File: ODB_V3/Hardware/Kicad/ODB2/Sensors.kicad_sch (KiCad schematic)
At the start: 24 parts, among them J4 RF2-04A-T-00-50-G, U10 ADXL382-2BCCZ-RL7, U4 MS580301BA01-00, U5 L76L-M33, U6 BNO055, U9 MAX6612MXK

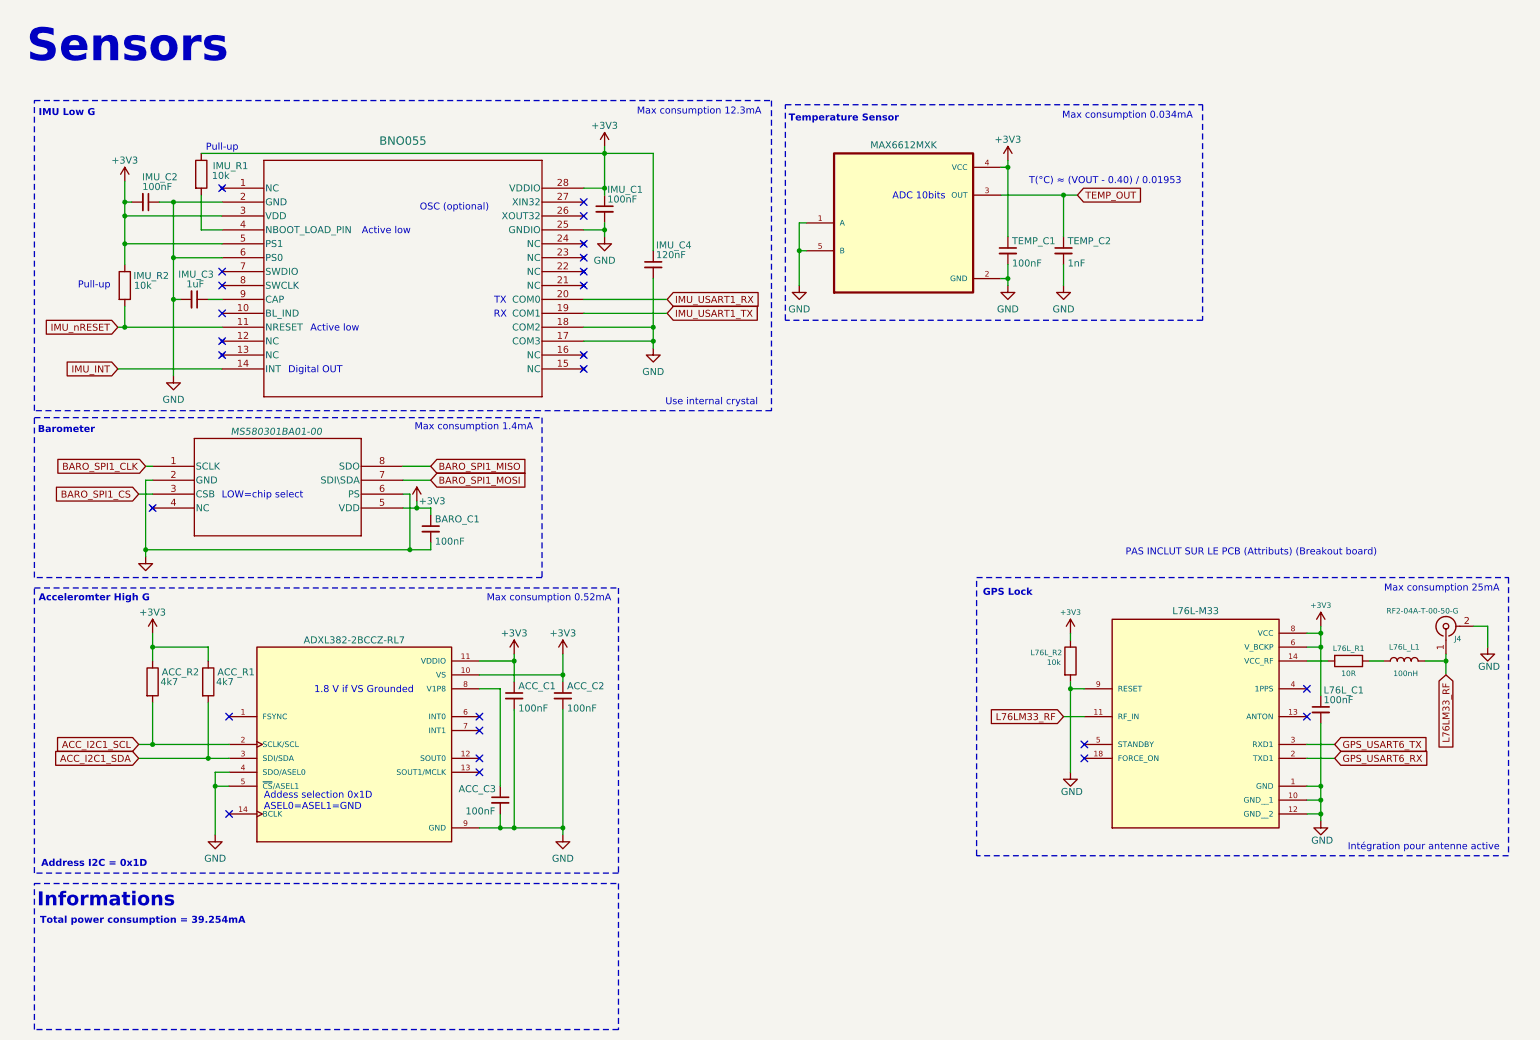
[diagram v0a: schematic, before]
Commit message: fix: labels
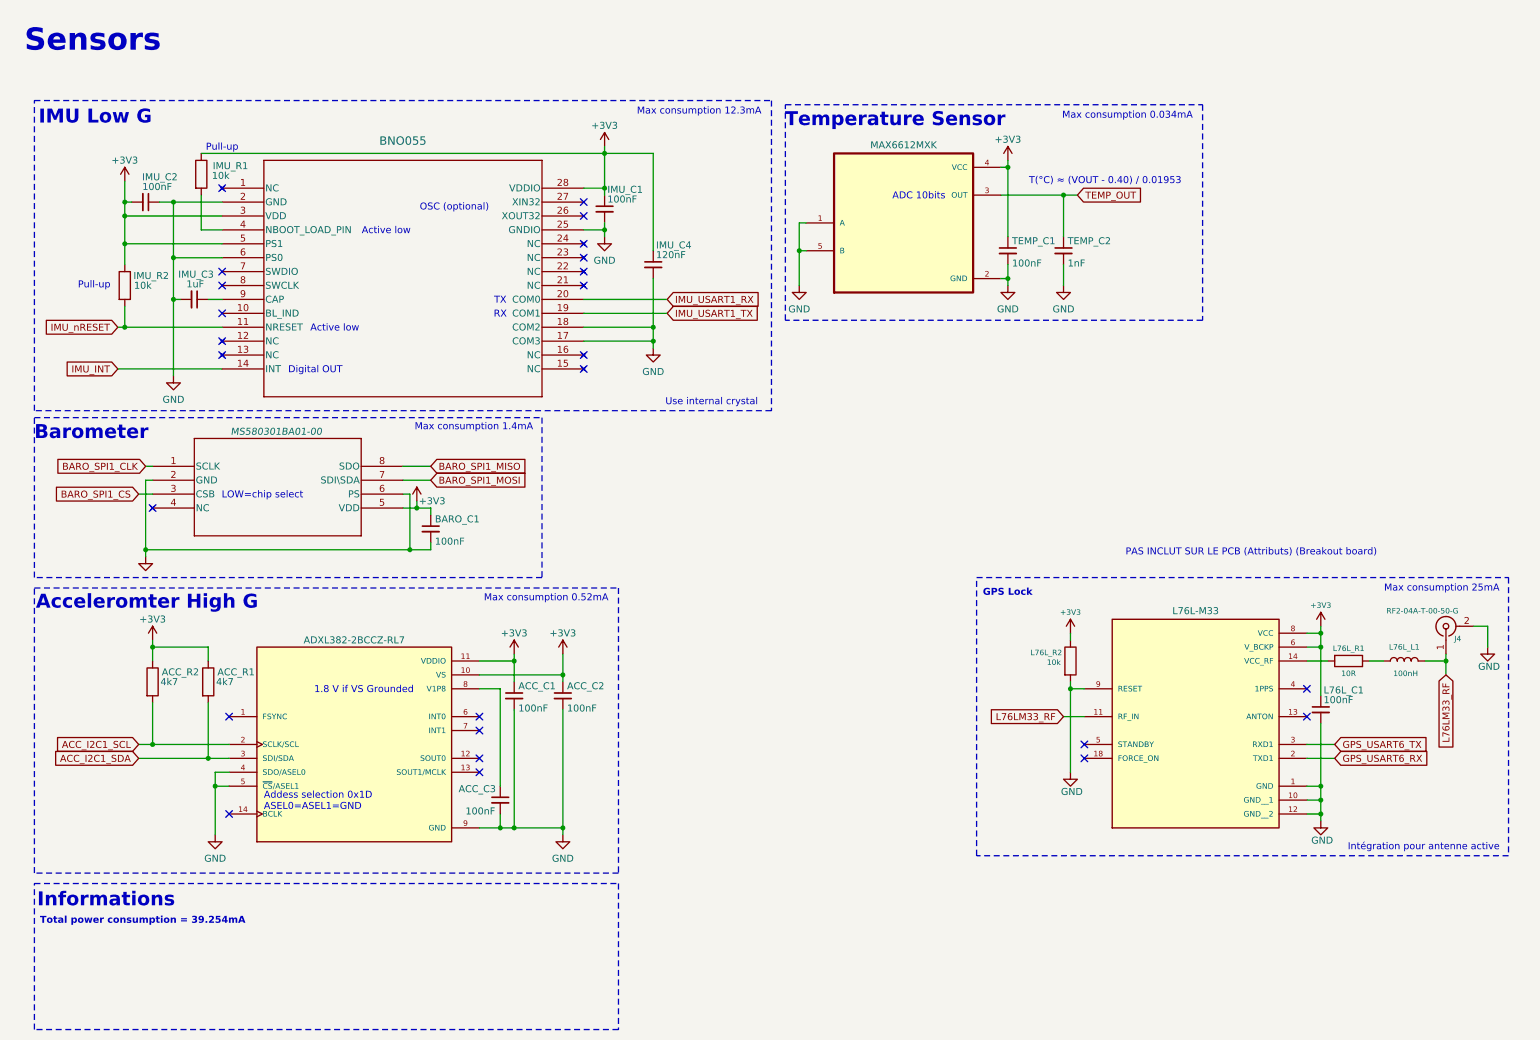
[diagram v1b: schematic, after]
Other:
- note removed: "Address I2C = 0x1D"
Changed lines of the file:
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@@
 	(text "Max consumption 0.52mA"
 		(exclude_from_sim no)
-		(at 107.95 118.11 0)
+		(at 107.442 118.11 0)
 		(effects
 			(font
@@
 	(text "Temperature Sensor"
 		(exclude_from_sim no)
-		(at 161.798 30.48 0)
+		(at 171.196 30.734 0)
 		(effects
 			(font
-				(size 1.27 1.27)
+				(size 2.54 2.54)
 				(thickness 0.254)
 				(bold yes)
@@
 		)
 	)
-	(text "Address I2C = 0x1D"
-		(exclude_from_sim no)
-		(at 24.892 166.624 0)
-		(effects
-			(font
-				(size 1.27 1.27)
-				(thickness 0.254)
-				(bold yes)
-			)
-		)
-	)
 	(text "Intégration pour antenne active"
 		(exclude_from_sim no)
@@
 	(text "Sensors"
 		(exclude_from_sim no)
-		(at 30.988 17.272 0)
+		(at 24.638 16.256 0)
 		(effects
 			(font
-				(size 6 6)
+				(size 4.064 4.064)
 				(thickness 0.254)
 				(bold yes)
@@
 	(text "Acceleromter High G"
 		(exclude_from_sim no)
-		(at 24.892 118.11 0)
+		(at 34.544 118.872 0)
 		(effects
 			(font
-				(size 1.27 1.27)
+				(size 2.54 2.54)
 				(thickness 0.254)
 				(bold yes)
@@
 	(text "Barometer"
 		(exclude_from_sim no)
-		(at 19.812 87.376 0)
+		(at 24.384 87.884 0)
 		(effects
 			(font
-				(size 1.27 1.27)
+				(size 2.54 2.54)
 				(thickness 0.254)
 				(bold yes)
@@
 	(text "IMU Low G"
 		(exclude_from_sim no)
-		(at 14.732 30.226 0)
+		(at 14.732 31.75 0)
 		(effects
 			(font
-				(size 1.27 1.27)
+				(size 2.54 2.54)
 				(thickness 0.254)
 				(bold yes)
@@
 	(wire
 		(pts
+			(xy 35.56 125.73) (xy 35.56 127)
+		)
+		(stroke
+			(width 0)
+			(type default)
+		)
+	)
+	(wire
+		(pts
 			(xy 246.38 129.54) (xy 250.19 129.54)
 		)
@@
 	(wire
 		(pts
-			(xy 35.56 124.46) (xy 35.56 127)
-		)
-		(stroke
-			(width 0)
-			(type default)
-		)
-	)
-	(wire
-		(pts
 			(xy 110.49 160.02) (xy 101.6 160.02)
 		)
@@
 	(symbol
 		(lib_id "power:+3V3")
-		(at 35.56 124.46 0)
+		(at 35.56 125.73 0)
 		(unit 1)
 		(exclude_from_sim no)
@@
 		(dnp no)
 		(property "Reference" "#PWR088"
-			(at 35.56 128.27 0)
+			(at 35.56 129.54 0)
 			(effects
 				(font
@@
 		)
 		(property "Value" "+3V3"
-			(at 35.56 120.65 0)
+			(at 35.56 121.92 0)
 			(effects
 				(font
@@
 		)
 		(property "Footprint" ""
-			(at 35.56 124.46 0)
+			(at 35.56 125.73 0)
 			(effects
 				(font
@@
 		)
 		(property "Datasheet" ""
-			(at 35.56 124.46 0)
+			(at 35.56 125.73 0)
 			(effects
 				(font
@@
 		)
 		(property "Description" "Power symbol creates a global label with name \"+3V3\""
-			(at 35.56 124.46 0)
+			(at 35.56 125.73 0)
 			(effects
 				(font
